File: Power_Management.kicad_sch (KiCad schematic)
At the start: 17 parts, among them J2 I2S_OR_LJ_OUT, Q1 MOSFET_SI2333DDS-T1-BE3

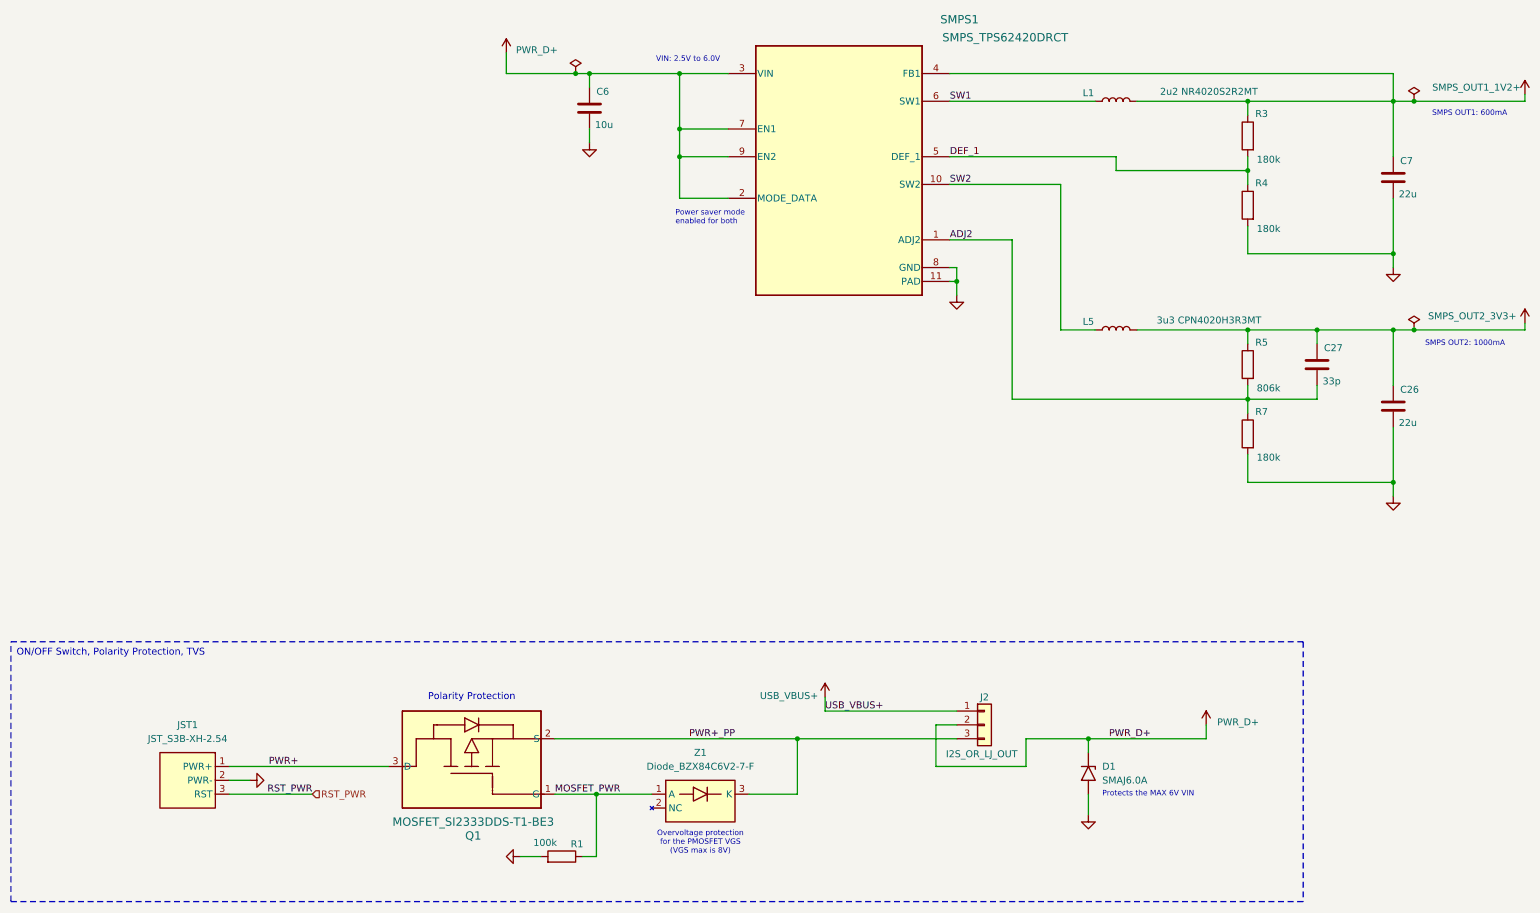
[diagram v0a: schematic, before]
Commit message: Update
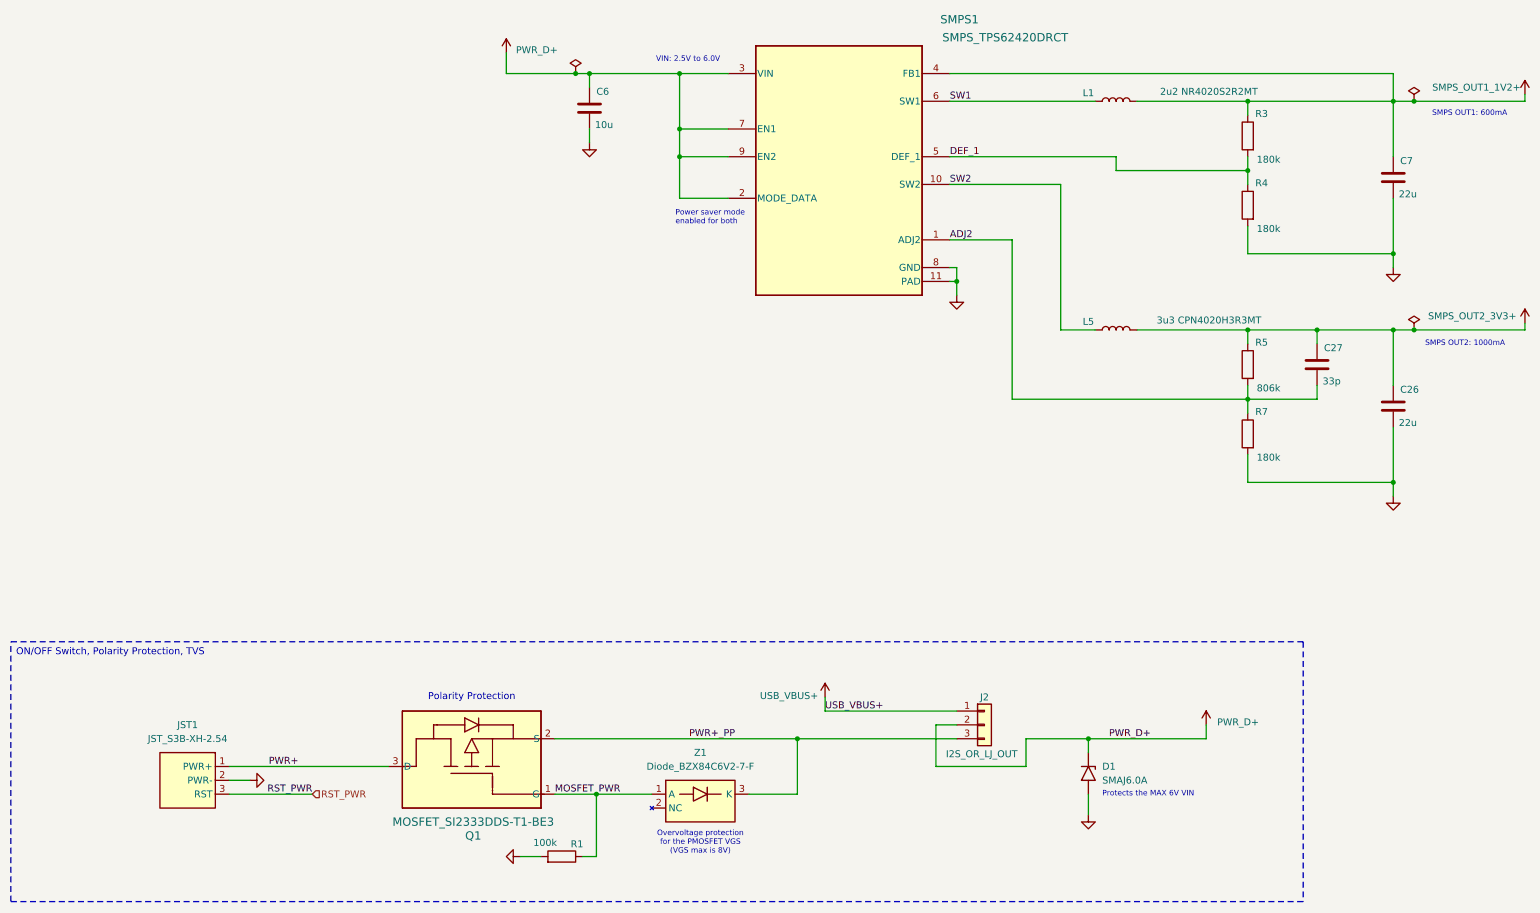
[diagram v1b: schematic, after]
